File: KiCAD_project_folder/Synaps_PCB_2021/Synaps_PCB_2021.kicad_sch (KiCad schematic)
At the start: 0 parts

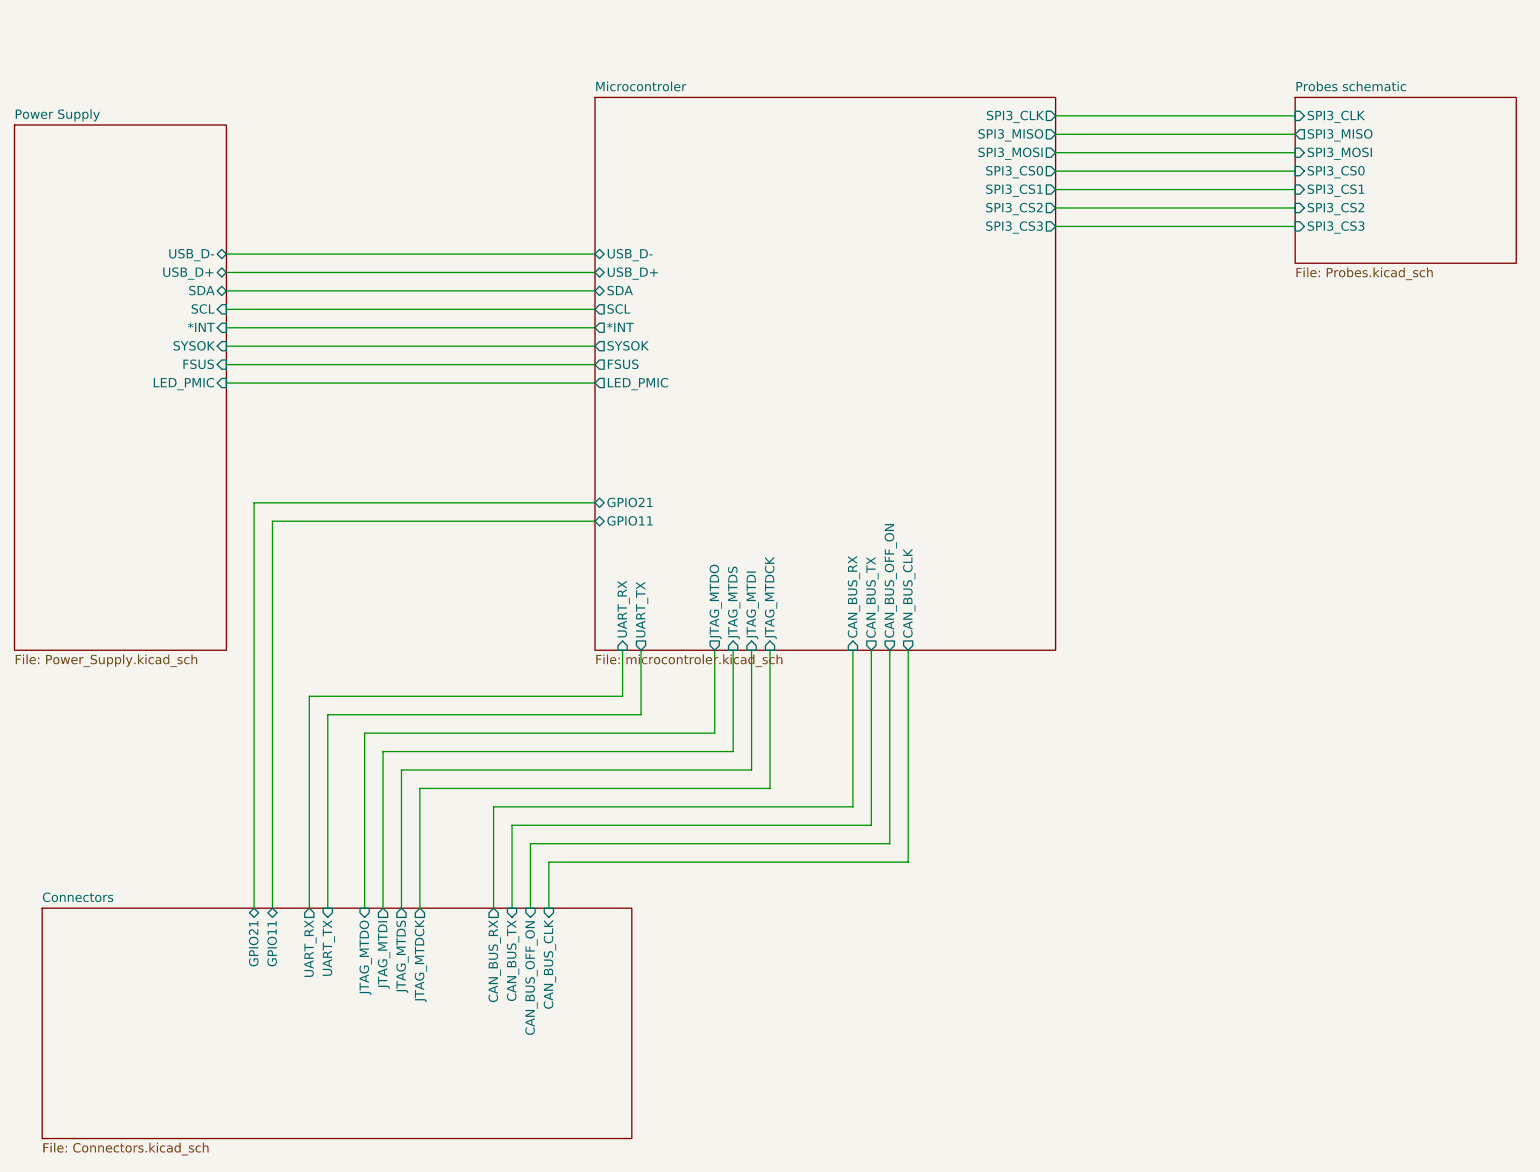
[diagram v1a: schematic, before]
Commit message: wip
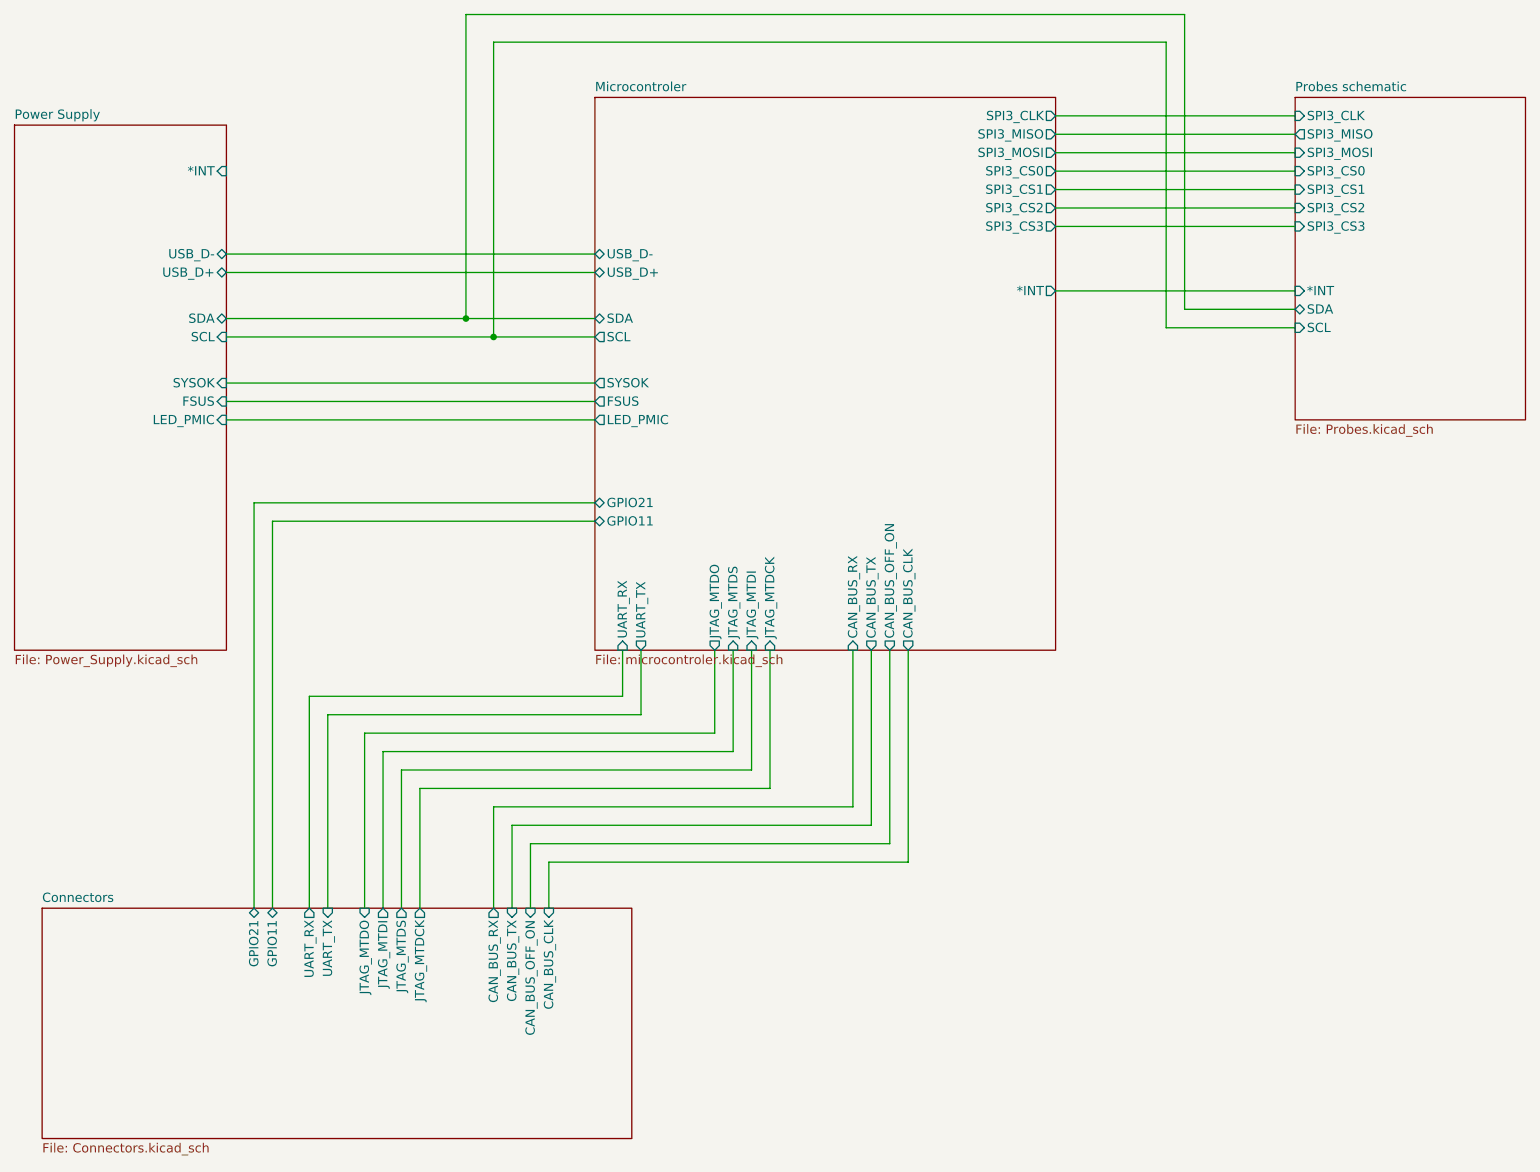
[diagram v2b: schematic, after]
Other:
- sheet Probes schematic ports: added *INT, SCL, SDA; removed none
